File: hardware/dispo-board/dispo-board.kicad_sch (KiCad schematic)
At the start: 32 parts, among them SW1 SW_Push, U1 TPS79633DCQ, U2 STM32H725RGV6, Y1 32M

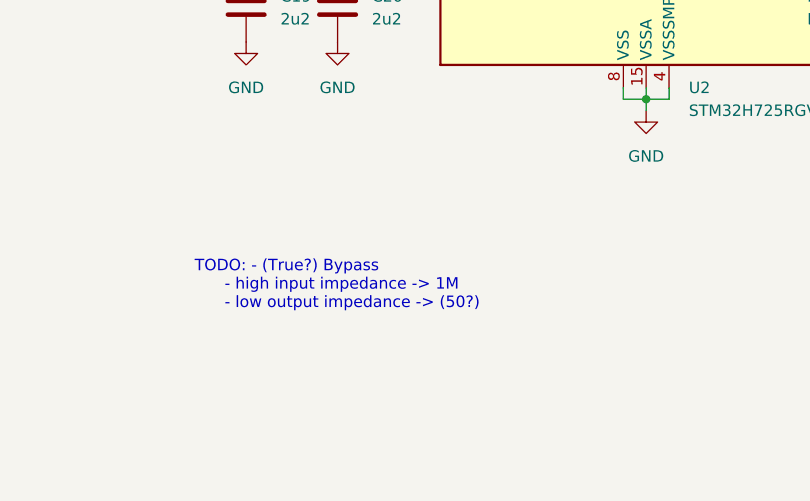
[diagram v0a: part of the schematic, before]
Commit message: maybe final schematic?
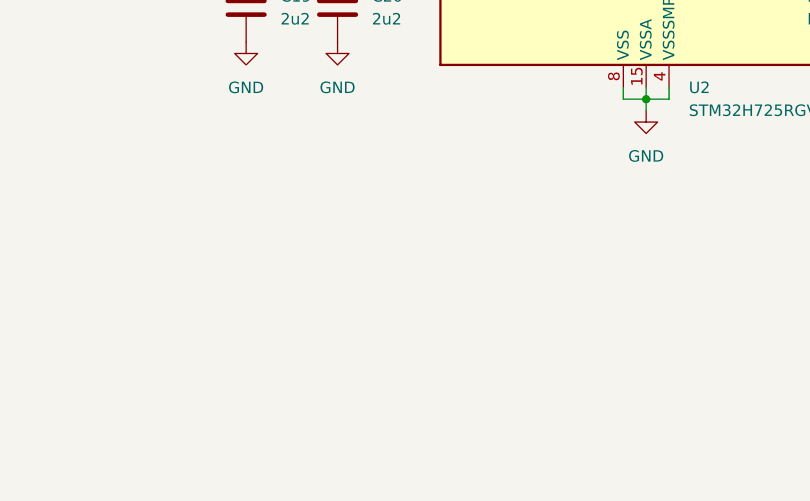
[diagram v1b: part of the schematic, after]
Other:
- note removed: "TODO: - (True?) Bypass - high input impedance -> 1M - low output impedance -> (50?)"
